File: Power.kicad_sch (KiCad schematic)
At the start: 35 parts, among them IC3 NCV8165ML330TCG, IC4 CYPD3177-24LQXQ, J1 USB_C_Receptacle_PowerOnly_6P, Q7 IRF9358TRPBF, Q8 IRF9358TRPBF, Q9 BSL308PEH6327XTSA1

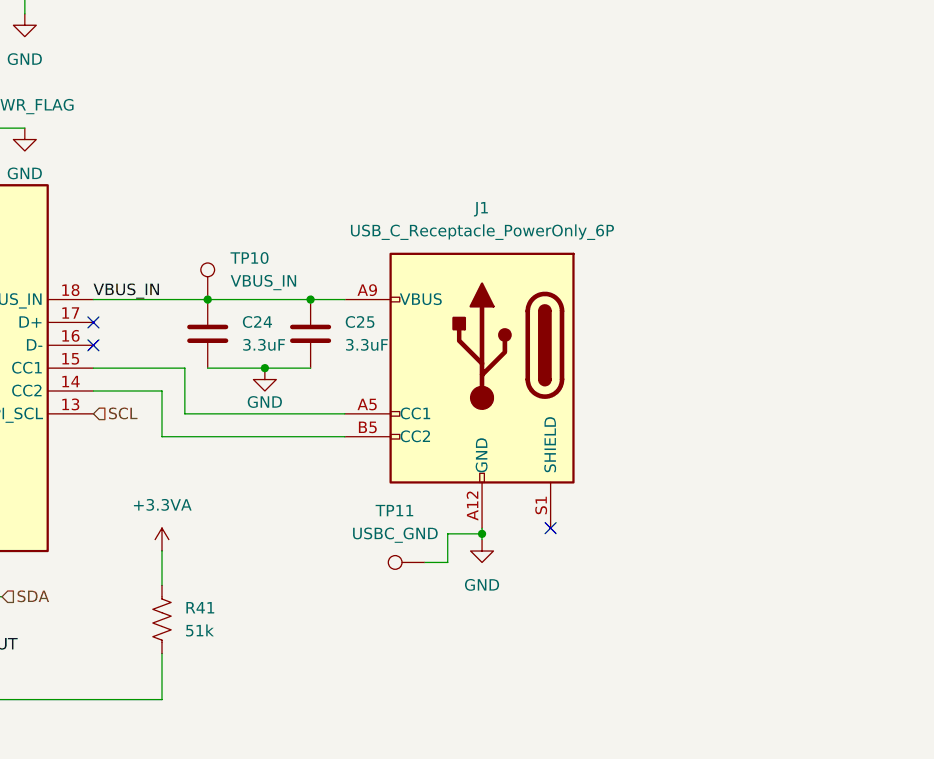
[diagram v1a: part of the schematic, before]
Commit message: updated footprints and started tracing
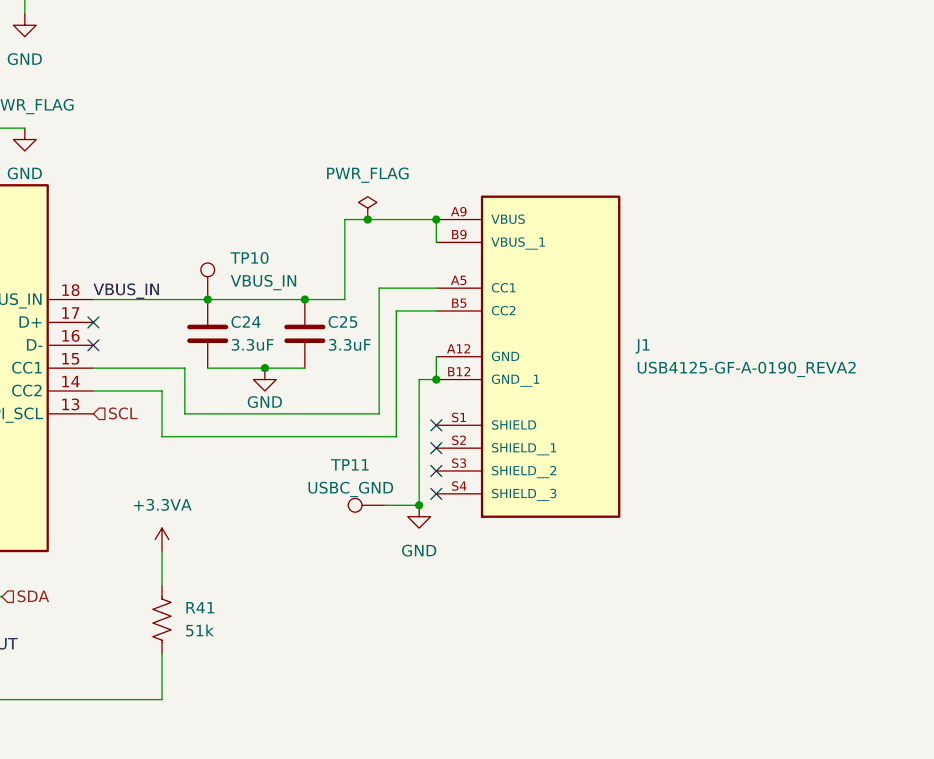
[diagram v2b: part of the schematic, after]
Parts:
- removed J1: USB_C_Receptacle_PowerOnly_6P, Connector_USB:USB_C_Receptacle_HCTL_HC-TYPE-C-16P-01A, symbol Connector:USB_C_Receptacle_PowerOnly_6P
- added J1: USB4125-GF-A-0190_REVA2, ExternalFootprints:GCT_USB4125-GF-A-0190_REVA2, symbol USB4125-GF-A-0190_REVA2:USB4125-GF-A-0190_REVA2
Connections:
- net GND: now also J1.A12 (GND), J1.B12 (GND__1)
- net VBUS_IN: now also J1.A9 (VBUS), J1.B9 (VBUS__1)
- net at IC4.14 (CC2): now also J1.B5 (CC2)
- net at IC4.15 (CC1): now also J1.A5 (CC1)
- no-connect marks 10 -> 13
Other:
- moved on the sheet: C25, TP11
